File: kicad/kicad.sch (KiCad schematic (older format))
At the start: 57 parts, among them J1 USB_B_Micro, J2 debug, J3 spi, J4 i2c, J5 led_front, J6 led_back, Q1 SI2365EDS-T1-GE3, Q2 2N7002, SW1 SW_Reed, SW2 Rotary_Encoder_Switch, SW3 SW_Push, U1 MCP73831-2-OT, U2 STM32L152R6HxA, U3 MIC2288YD5, U4 BD70522GUL-E2

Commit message: version updates
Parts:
- J1: symbol Connector:USB_B_Micro -> kicad-rescue:USB_B_Micro-Connector
- LCD1: symbol good_things:LCD-S2X1C50TR -> kicad-rescue:LCD-S2X1C50TR-good_things
- U3: symbol good_things:MIC2288YD5 -> kicad-rescue:MIC2288YD5-good_things
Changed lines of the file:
@@
 	4100 2150 4100 2350
 $Comp
-L good_things:LCD-S2X1C50TR LCD1
+L kicad-rescue:LCD-S2X1C50TR-good_things LCD1
 U 1 1 60C40D31
 P 9500 1500
@@
 NoConn ~ 1000 2350
 $Comp
-L Connector:USB_B_Micro J1
+L kicad-rescue:USB_B_Micro-Connector J1
 U 1 1 60BEF3CC
 P 1100 1950
@@
 vbus
 $Comp
-L good_things:MIC2288YD5 U3
+L kicad-rescue:MIC2288YD5-good_things U3
 U 1 1 60CAF0CF
 P 5650 2450

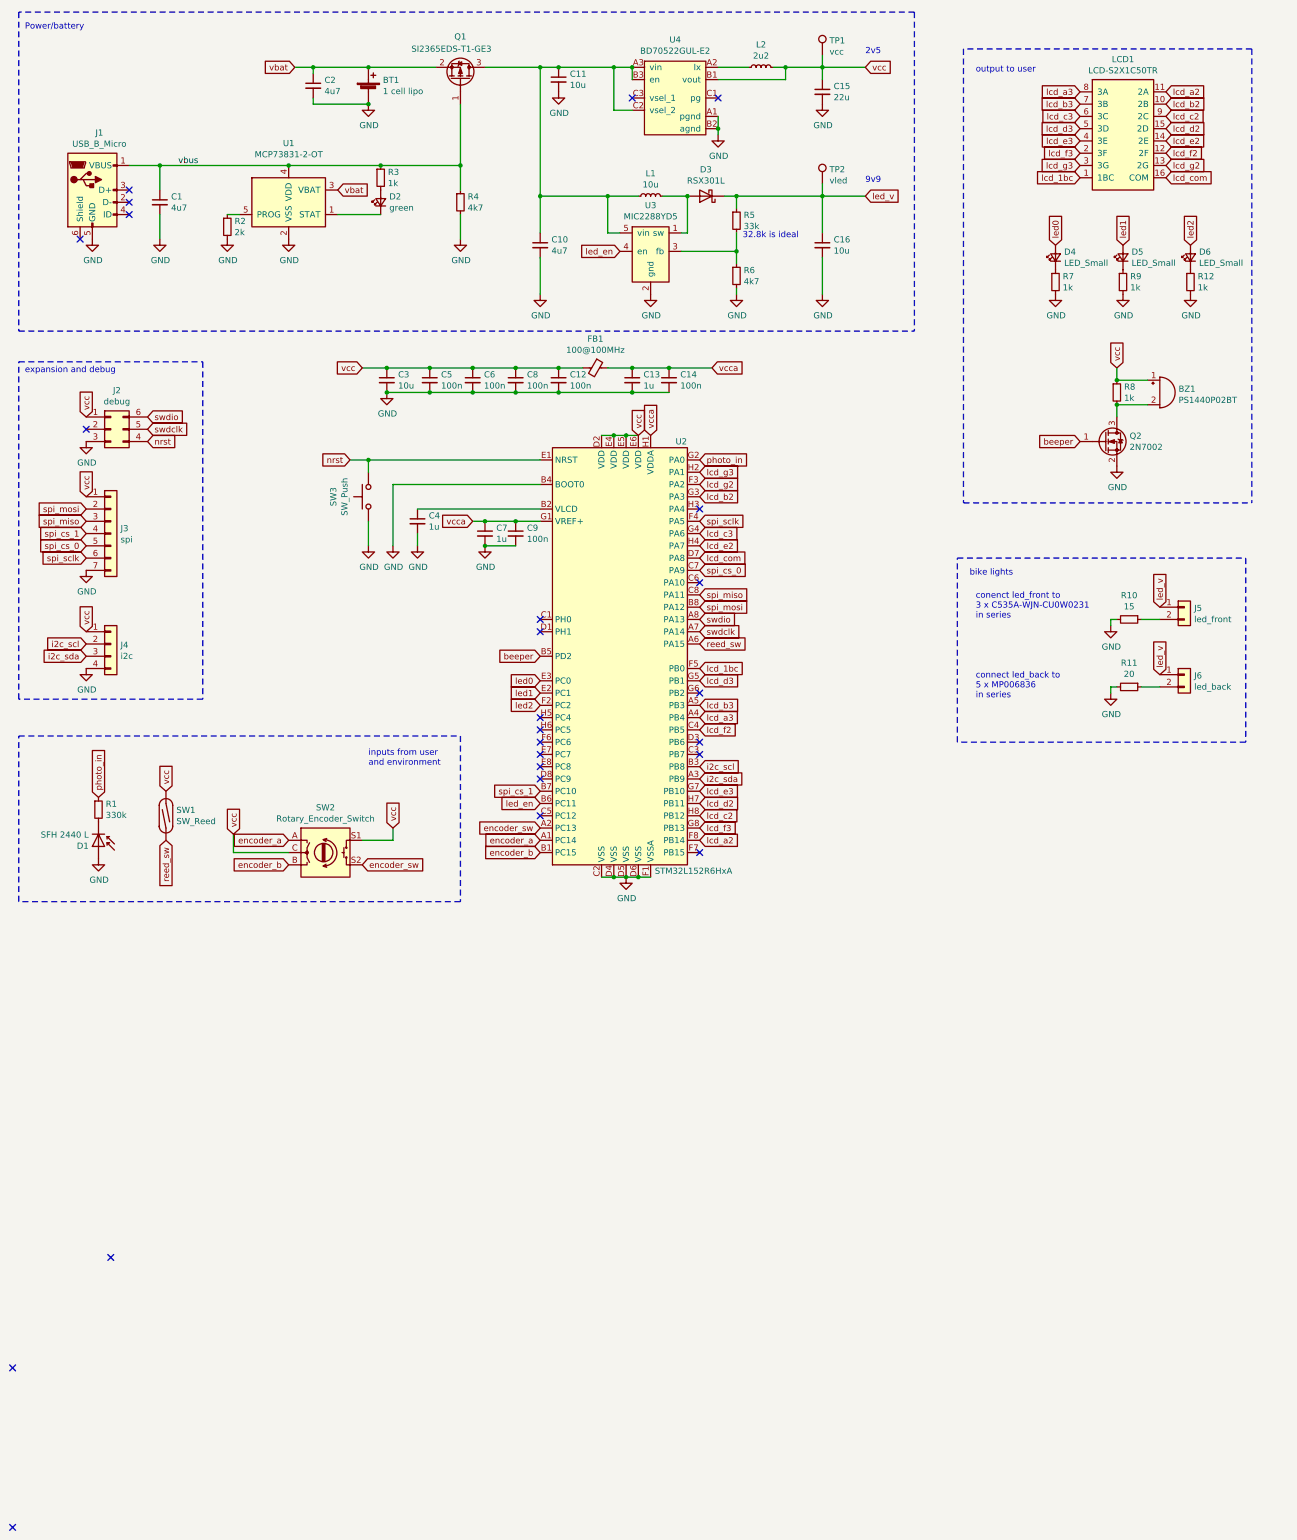
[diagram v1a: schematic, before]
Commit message: Some schema work with correct mcu
also rm some shit
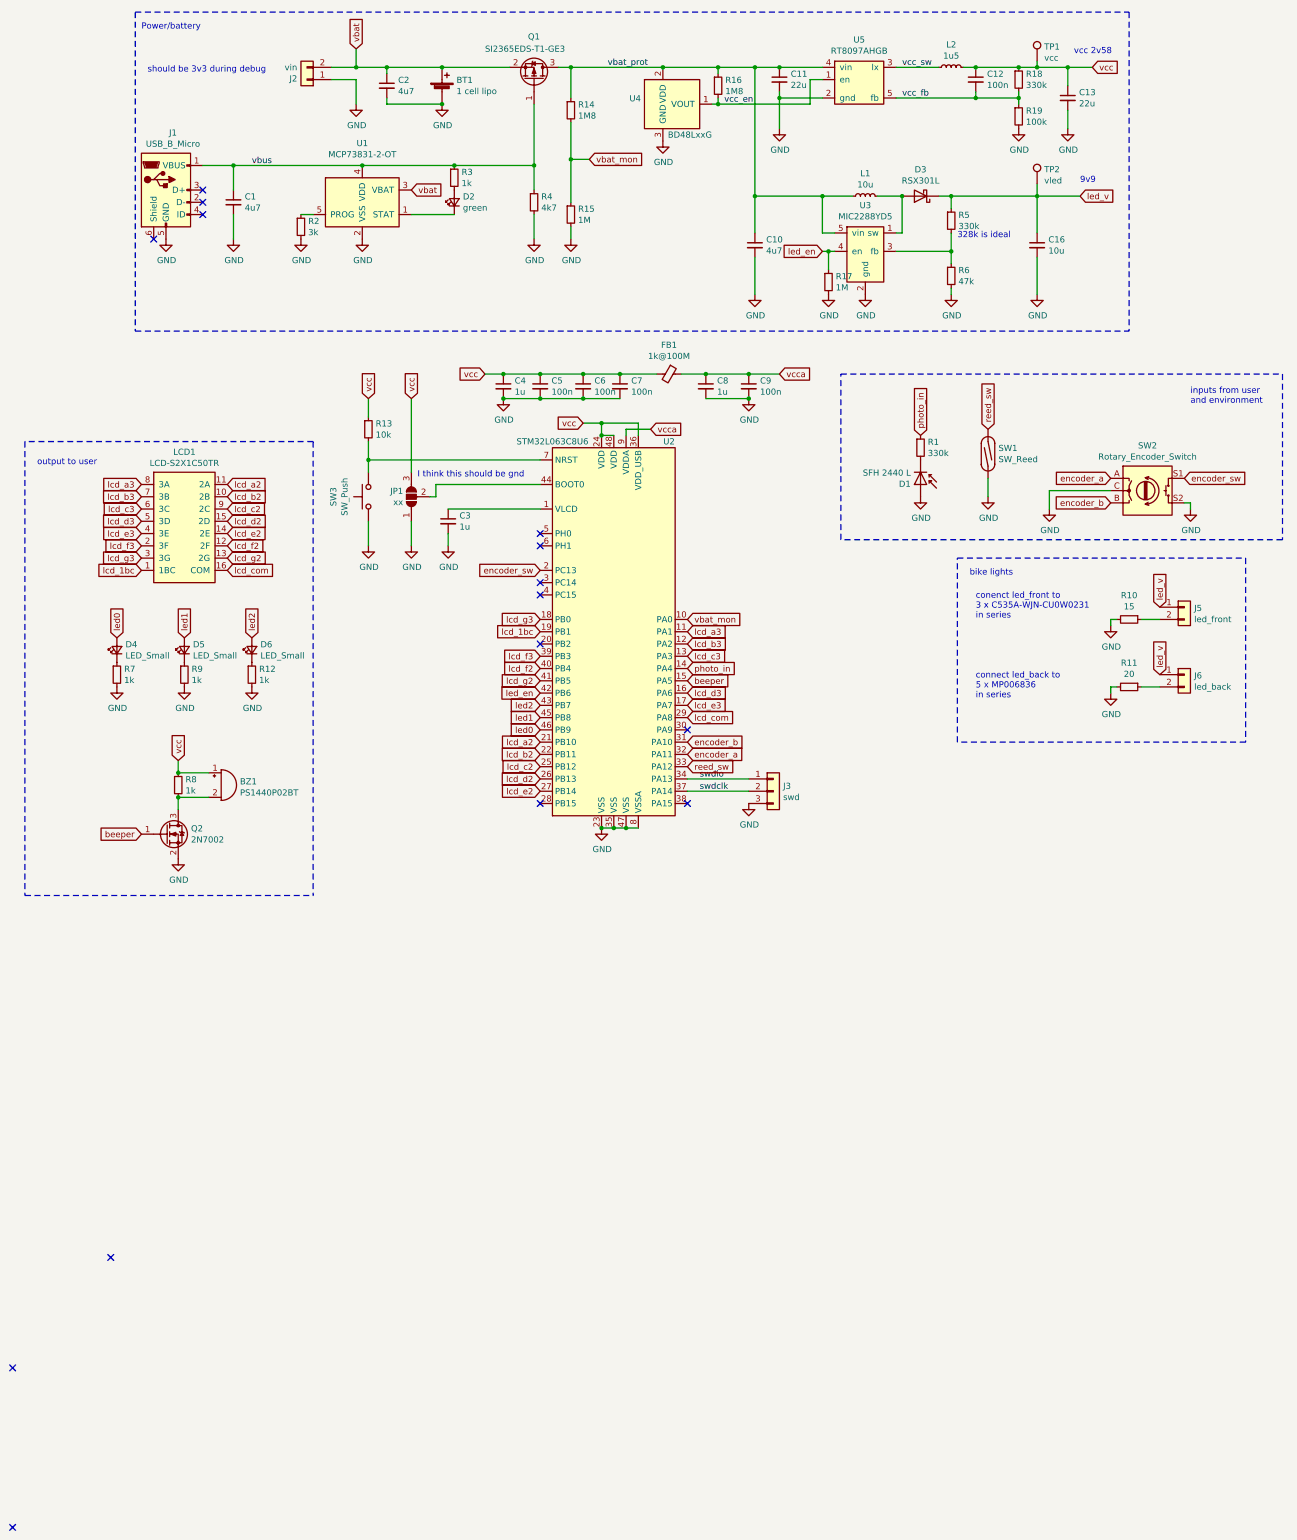
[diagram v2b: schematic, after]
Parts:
- removed C14: 100n, symbol Device:C_Small
- removed C15: 22u, symbol Device:C_Small
- removed J2: debug, symbol Connector_Generic:Conn_02x03_Counter_Clockwise
- removed J3: spi, symbol Connector_Generic:Conn_01x07
- removed J4: i2c, symbol Connector_Generic:Conn_01x04
- removed U2: STM32L152R6HxA, Package_BGA:TFBGA-64_5x5mm_Layout8x8_P0.5mm, symbol MCU_ST_STM32L1:STM32L152R6HxA
- removed U4: BD70522GUL-E2, symbol good_things:BD70522GUL-E2
- added J2: vin, Connector_Phoenix_MSTB:PhoenixContact_MSTBVA_2,5_2-G_1x02_P5.00mm_Vertical, symbol Connector_Generic:Conn_01x02
- added J3: swd, Connector_PinHeader_2.54mm:PinHeader_1x03_P2.54mm_Vertical, symbol Connector_Generic:Conn_01x03
- added JP1: xx, Jumper:SolderJumper-3_P1.3mm_Open_Pad1.0x1.5mm, symbol Jumper:SolderJumper_3_Open
- added R13: 10k, Resistor_SMD:R_0603_1608Metric_Pad0.98x0.95mm_HandSolder, symbol Device:R_Small
- added R14, R16: 1M8, Resistor_SMD:R_0603_1608Metric_Pad0.98x0.95mm_HandSolder, symbol Device:R_Small
- added R15, R17: 1M, Resistor_SMD:R_0603_1608Metric_Pad0.98x0.95mm_HandSolder, symbol Device:R_Small
- added R18: 330k, Resistor_SMD:R_0603_1608Metric_Pad0.98x0.95mm_HandSolder, symbol Device:R_Small
- added R19: 100k, Resistor_SMD:R_0603_1608Metric_Pad0.98x0.95mm_HandSolder, symbol Device:R_Small
- added U2: STM32L063C8U6, Package_QFP:LQFP-48_7x7mm_P0.5mm, symbol MCU_ST_STM32L0:STM32L063C8Tx
- added U4: BD48LxxG, Package_TO_SOT_SMD:SOT-23, symbol Power_Management:BD48LxxG
- added U5: RT8097AHGB, Package_TO_SOT_SMD:SOT-23-5_HandSoldering, symbol good_things:RT8097AHGB
- C1, C10, C12, C16, C2, C4, C5, C6, C9: footprint (none) -> Capacitor_SMD:C_0603_1608Metric_Pad1.08x0.95mm_HandSolder
- C11: value 10u -> 22u; footprint (none) -> Capacitor_SMD:C_0603_1608Metric_Pad1.08x0.95mm_HandSolder
- C13: value 1u -> 22u; footprint (none) -> Capacitor_SMD:C_0603_1608Metric_Pad1.08x0.95mm_HandSolder
- C3: value 10u -> 1u; footprint (none) -> Capacitor_SMD:C_0603_1608Metric_Pad1.08x0.95mm_HandSolder
- C7: value 1u -> 100n; footprint (none) -> Capacitor_SMD:C_0603_1608Metric_Pad1.08x0.95mm_HandSolder
- C8: value 100n -> 1u; footprint (none) -> Capacitor_SMD:C_0603_1608Metric_Pad1.08x0.95mm_HandSolder
- D1: footprint (none) -> good_things:sfh-2440-l
- D2, D4, D5, D6: footprint (none) -> LED_SMD:LED_0603_1608Metric_Pad1.05x0.95mm_HandSolder
- D3: footprint (none) -> good_things:SOD-106
- FB1: value 100@100MHz -> 1k@100M; footprint (none) -> Inductor_SMD:L_0603_1608Metric_Pad1.05x0.95mm_HandSolder
- J1: footprint (none) -> good_things:USB_MICRO_10118193-0001LF
- J5, J6, SW1: footprint (none) -> Connector_Phoenix_MSTB:PhoenixContact_MSTBVA_2,5_2-G_1x02_P5.00mm_Vertical
- L2: value 2u2 -> 1u5; footprint (none) -> Inductor_SMD:L_Sunlord_MWSA0518_5.4x5.2mm
- R1, R10, R11, R12, R3, R4, R7, R8, R9: footprint (none) -> Resistor_SMD:R_0603_1608Metric_Pad0.98x0.95mm_HandSolder
- R2: value 2k -> 3k; footprint (none) -> Resistor_SMD:R_0603_1608Metric_Pad0.98x0.95mm_HandSolder
- R5: value 33k -> 330k; footprint (none) -> Resistor_SMD:R_0603_1608Metric_Pad0.98x0.95mm_HandSolder
- R6: value 4k7 -> 47k; footprint (none) -> Resistor_SMD:R_0603_1608Metric_Pad0.98x0.95mm_HandSolder
- SW2: footprint (none) -> Rotary_Encoder:RotaryEncoder_Alps_EC11E_Vertical_H20mm
- SW3: footprint (none) -> good_things:push_sw_purple
- TP1, TP2: footprint (none) -> TestPoint:TestPoint_Pad_1.5x1.5mm
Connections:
- net GND: now also SW1.2, SW2.C, SW2.S2, J2.1 (Pin_1), J3.3 (Pin_3), JP1.1 (A), R15.2, R17.2, R19.2, U2.23 (VSS), U2.35 (VSS), U2.47 (VSS), U2.8 (VSSA), U4.3 (GND), U5.2 (gnd); no longer C12.2
- net beeper: now also U2.15 (PA5)
- net encoder_a: now also U2.32 (PA11)
- net encoder_b: now also U2.31 (PA10)
- net encoder_sw: now also SW2.S1, U2.2 (PC13); no longer SW2.S2
- net lcd_1bc: now also U2.19 (PB1)
- net lcd_a2: now also U2.21 (PB10)
- net lcd_a3: now also U2.11 (PA1)
- net lcd_b2: now also U2.22 (PB11)
- net lcd_b3: now also U2.12 (PA2)
- net lcd_c2: now also U2.25 (PB12)
- net lcd_c3: now also U2.13 (PA3)
- net lcd_com: now also U2.29 (PA8)
- net lcd_d2: now also U2.26 (PB13)
- net lcd_d3: now also U2.16 (PA6)
- net lcd_e2: now also U2.27 (PB14)
- net lcd_e3: now also U2.17 (PA7)
- net lcd_f2: now also U2.40 (PB4)
- net lcd_f3: now also U2.39 (PB3)
- net lcd_g2: now also U2.41 (PB5)
- net lcd_g3: now also U2.18 (PB0)
- net led0: now also U2.46 (PB9)
- net led1: now also U2.45 (PB8)
- net led2: now also U2.43 (PB7)
- net led_en: now also R17.1, U2.42 (PB6)
- net photo_in: now also U2.14 (PA4)
- net reed_sw: now also SW1.1, U2.33 (PA12); no longer SW1.2
- net swdclk: now also J3.2 (Pin_2), U2.37 (PA14)
- net swdio: now also J3.1 (Pin_1), U2.34 (PA13)
- net vbat: now also J2.2 (Pin_2)
- net vcc: now also C13.1, C4.1, C7.1, JP1.3 (B), R13.1, R18.1, U2.24 (VDD), U2.36 (VDD_USB), U2.48 (VDD); no longer C3.1, C8.1, SW1.1, SW2.C, SW2.S1
- net vcca: now also C8.1, U2.9 (VDDA); no longer C13.1, C7.1
- net vbat_prot: now reaches C10.1, C11.1, L1.1, Q1.3 (D), U3.5 (vin)
- net vbat_prot: now also R14.1, R16.1, U4.2 (VDD), U5.4 (vin)
- net vcc_sw: now reaches L2.1
- net vcc_sw: now also U5.3 (lx)
- net nrst: no longer names the net of SW3.2
- net nrst: now also R13.2, U2.7 (NRST)
- new net: C3.1, U2.1 (VLCD)
- new net: JP1.2 (C), U2.44 (BOOT0)
- new net vbat_mon: R14.2, R15.1, U2.10 (PA0)
- new net vcc_en: R16.2, U4.1 (VOUT), U5.1 (en)
- new net vcc_fb: C12.2, R18.2, R19.1, U5.5 (fb)
- no-connect marks 25 -> 15
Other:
- note added: "328k is ideal"
- note added: "I think this should be gnd"
- note added: "should be 3v3 during debug"
- note added: "vcc 2v58"
- note removed: "2v5"
- note removed: "32.8k is ideal"
- note removed: "expansion and debug"
- moved on the sheet: BT1, BZ1, C1, C10, C16, C2, D1, D2, D3, D4, D5, D6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
